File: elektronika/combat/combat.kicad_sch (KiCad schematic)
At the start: 35 parts, among them J1 odbiornik, J2 naped_prawy, J3 naped_lewy, J4 buzzer, J5 wyjscie do silnika +-, J6 Conn_02x04_Odd_Even, J7 zasilanie xt30, J8 Conn_01x01_Pin, J800 USB_C_Receptacle_USB2.0_16P, U1 ESP32-S3-WROOM-1, U2 kontroler_bldc, U3 AMS1117, U4 przetwornica

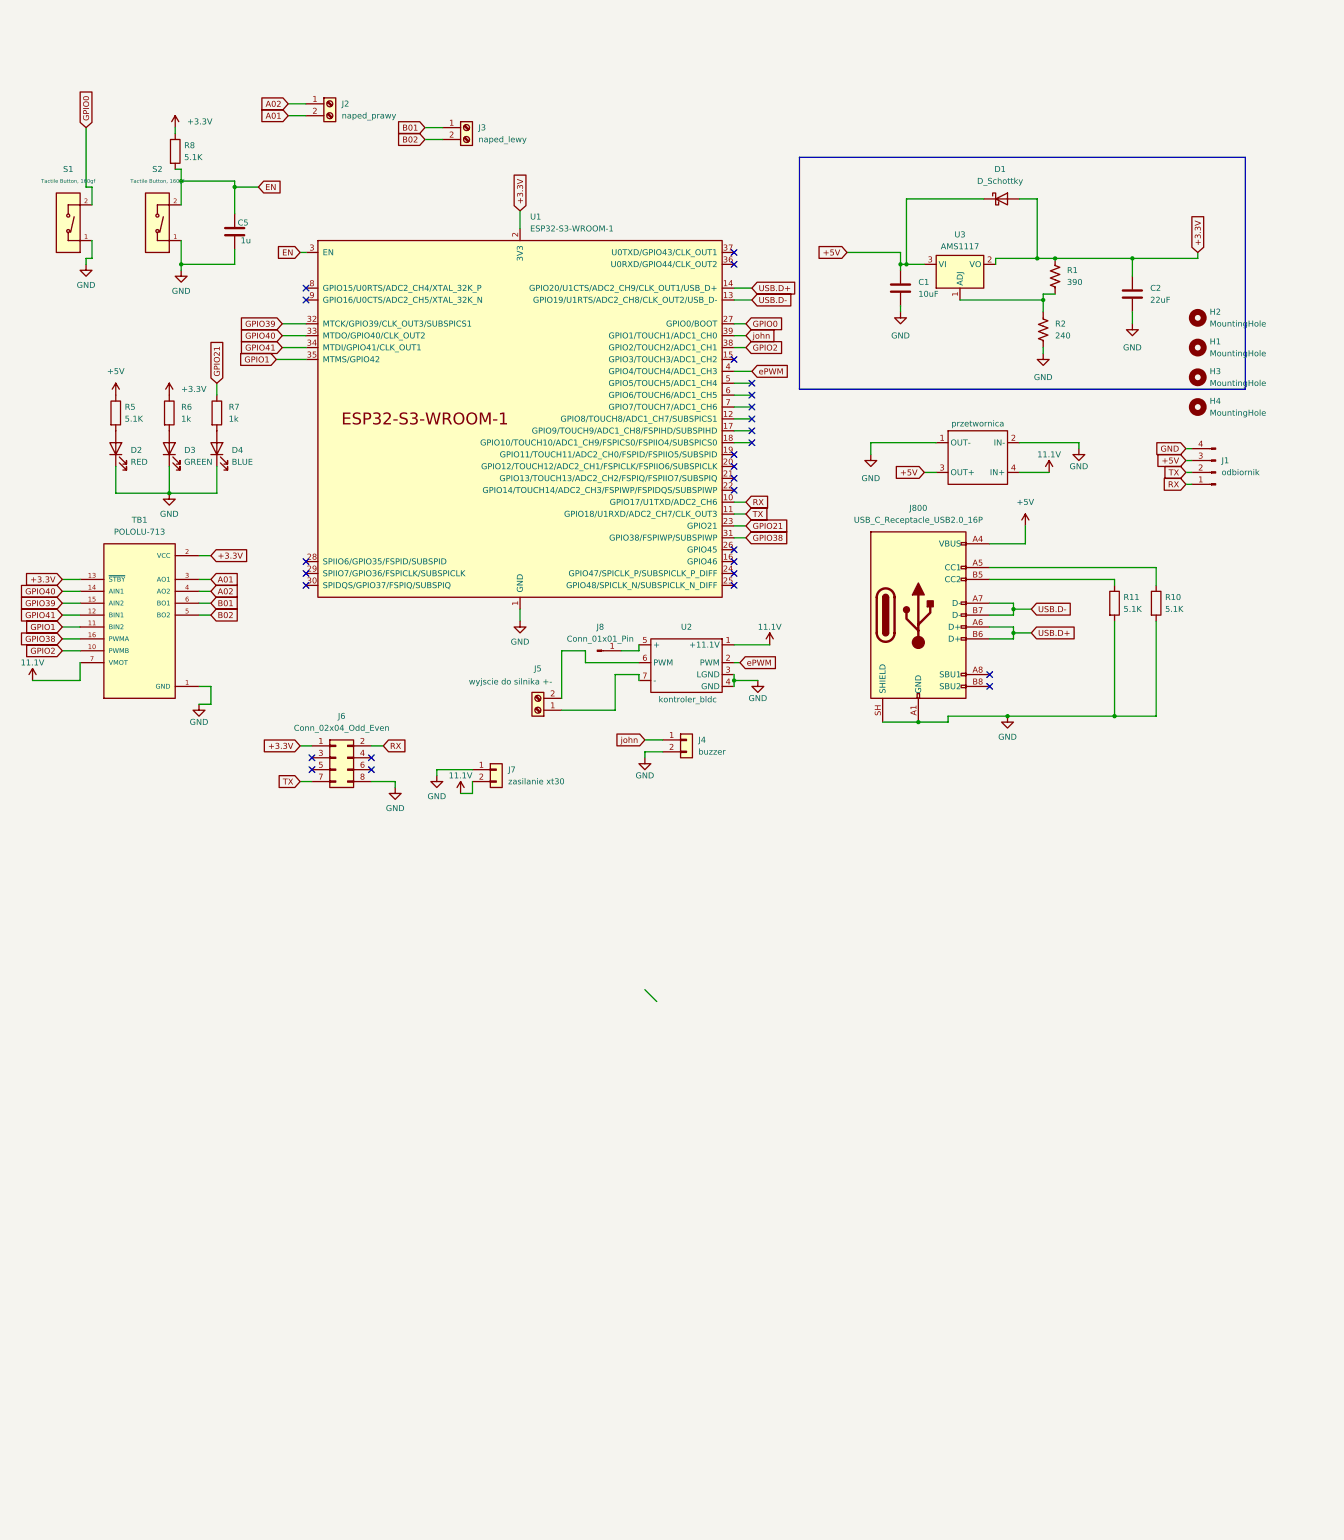
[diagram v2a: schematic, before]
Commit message: wersja nadajaca sie do sprawdzania
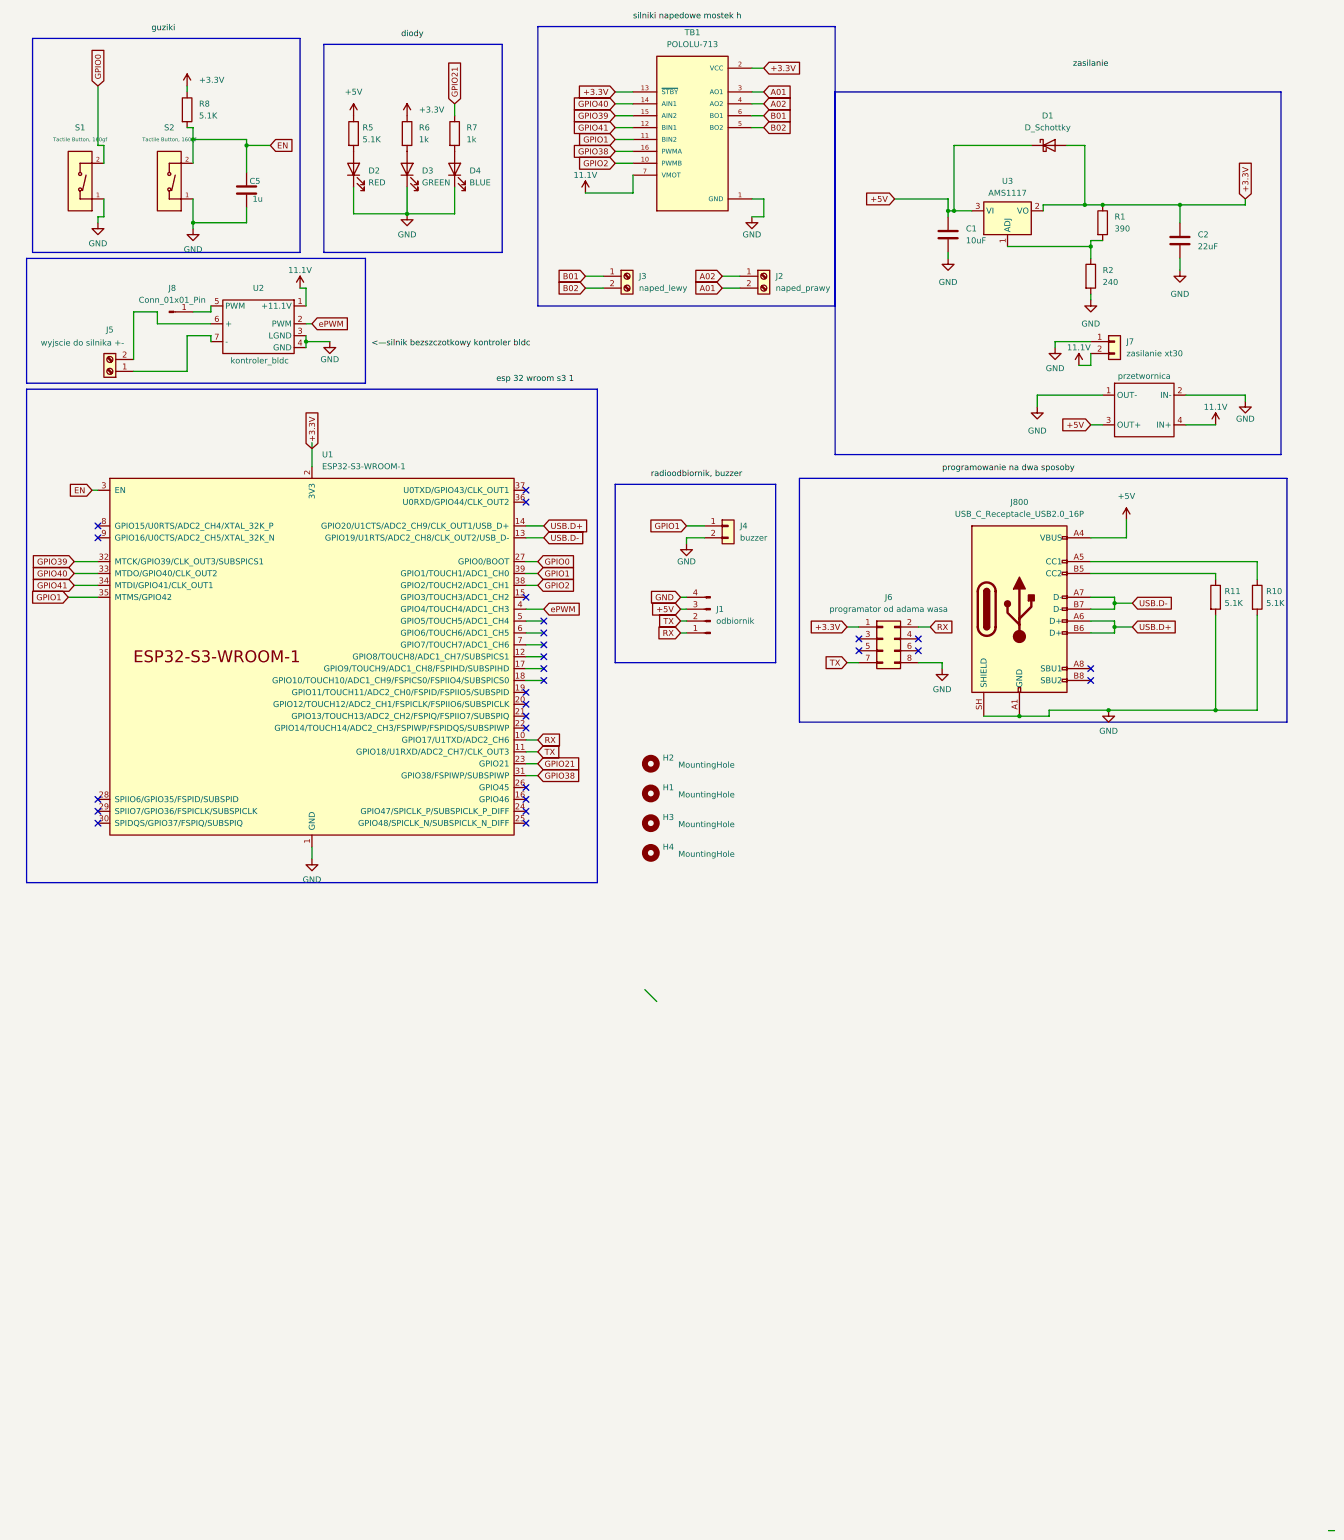
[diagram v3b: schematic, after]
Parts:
- removed R1: 390, PCM_SparkFun-Resistor:R_0603_1608Metric, symbol PCM_SparkFun-Resistor:R
- removed R2: 240, PCM_SparkFun-Resistor:R_0603_1608Metric, symbol PCM_SparkFun-Resistor:R
- added R1: 390, symbol Device:R
- added R2: 240, symbol Device:R
- J6: value Conn_02x04_Odd_Even -> programator od adama wasa
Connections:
- net john is gone; now on net GPIO1: J4.1 (Pin_1), U1.39 (GPIO1/TOUCH1/ADC1_CH0)
- net +3.3V: now also R1.1
- net GND: now also R2.2
- net at U3.1 (ADJ): now also R1.2, R2.1
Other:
- moved on the sheet: C1, C2, C5, D1, D2, D3, D4, H1, H2, H3, H4, J1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
